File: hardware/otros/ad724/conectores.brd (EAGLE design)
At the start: 24.1 x 39 mm, 5 parts, among them U1 MINI-DIN6PTH

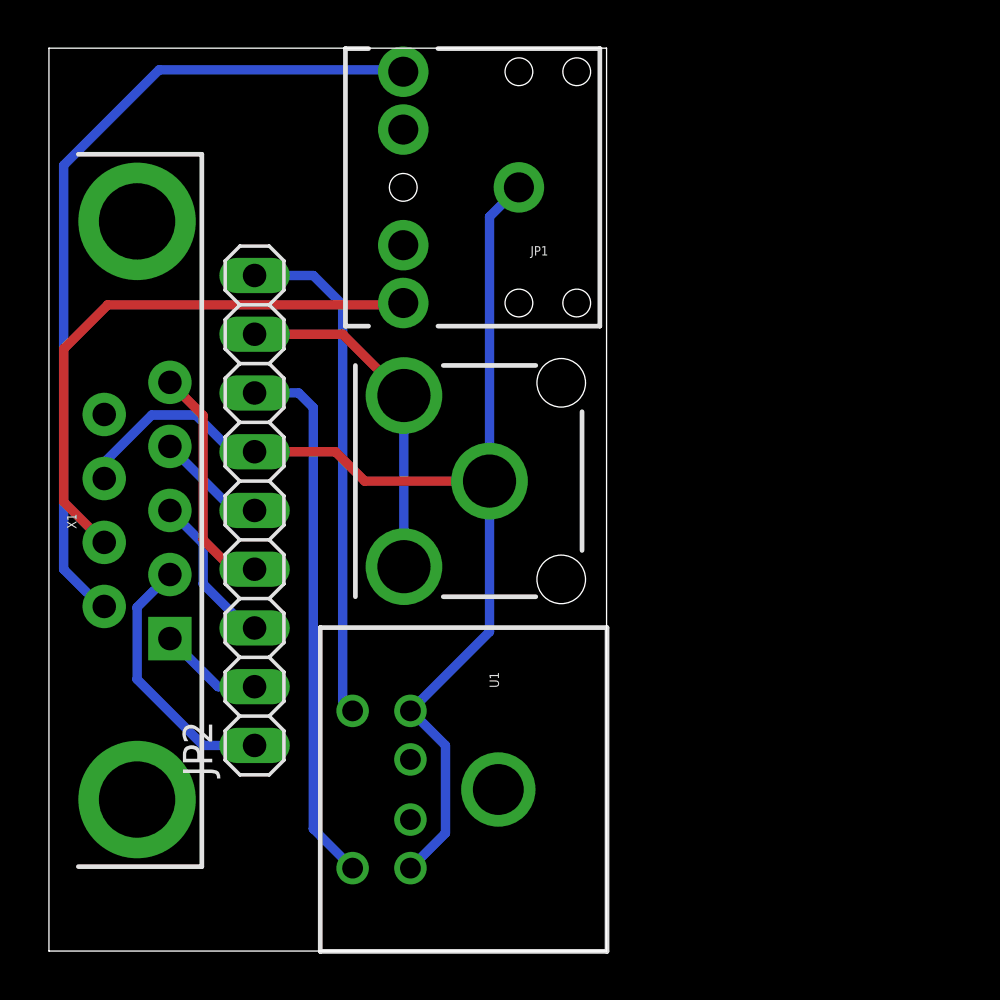
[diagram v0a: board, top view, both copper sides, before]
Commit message: planos de masa
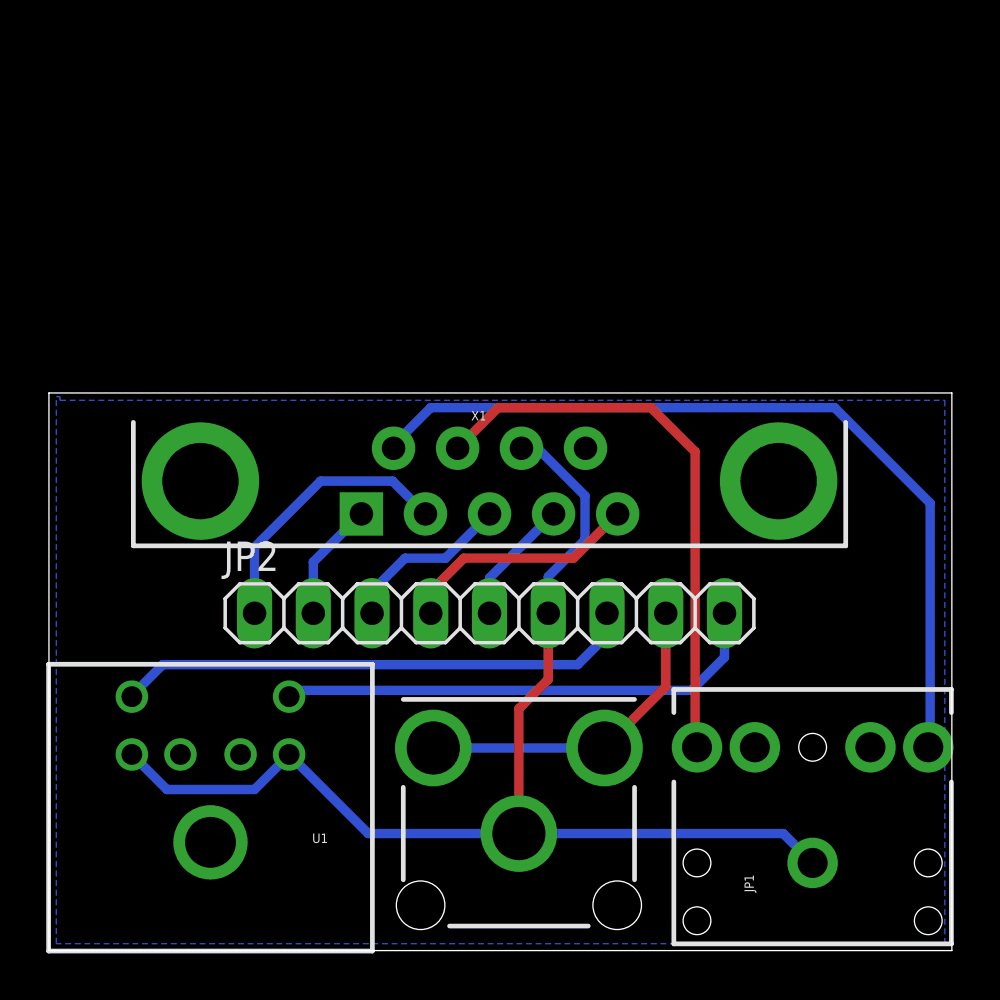
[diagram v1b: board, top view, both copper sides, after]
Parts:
- moved JP1 31.9 mm to (33.0, 3.81), turned to 90 degrees
- moved U1 18.5 mm to (6.99, 0.00), turned to 180 degrees
- moved JP3 15.3 mm to (20.3, 5.08), turned to 90 degrees
- moved X1 15.3 mm to (19.1, 20.3), turned to 0 degrees
- moved JP2 11.1 mm to (19.1, 14.6), turned to 0 degrees
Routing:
- net N$11: track 23.4 -> 22.6 mm
- net N$3: track 6.78 -> 7.42 mm
- net N$2: track 11.4 -> 12.0 mm
- net N$4: track 4.81 -> 5.44 mm
- net N$10: track 15.0 -> 14.3 mm
- net N$1: track 4.52 -> 5.16 mm
- net N$9: track 22.1 -> 21.4 mm
- added copper zone on layer 16, net GND
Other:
- board size 24.1 x 39 mm -> 39 x 24.1 mm
